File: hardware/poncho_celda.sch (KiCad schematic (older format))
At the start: 0 parts

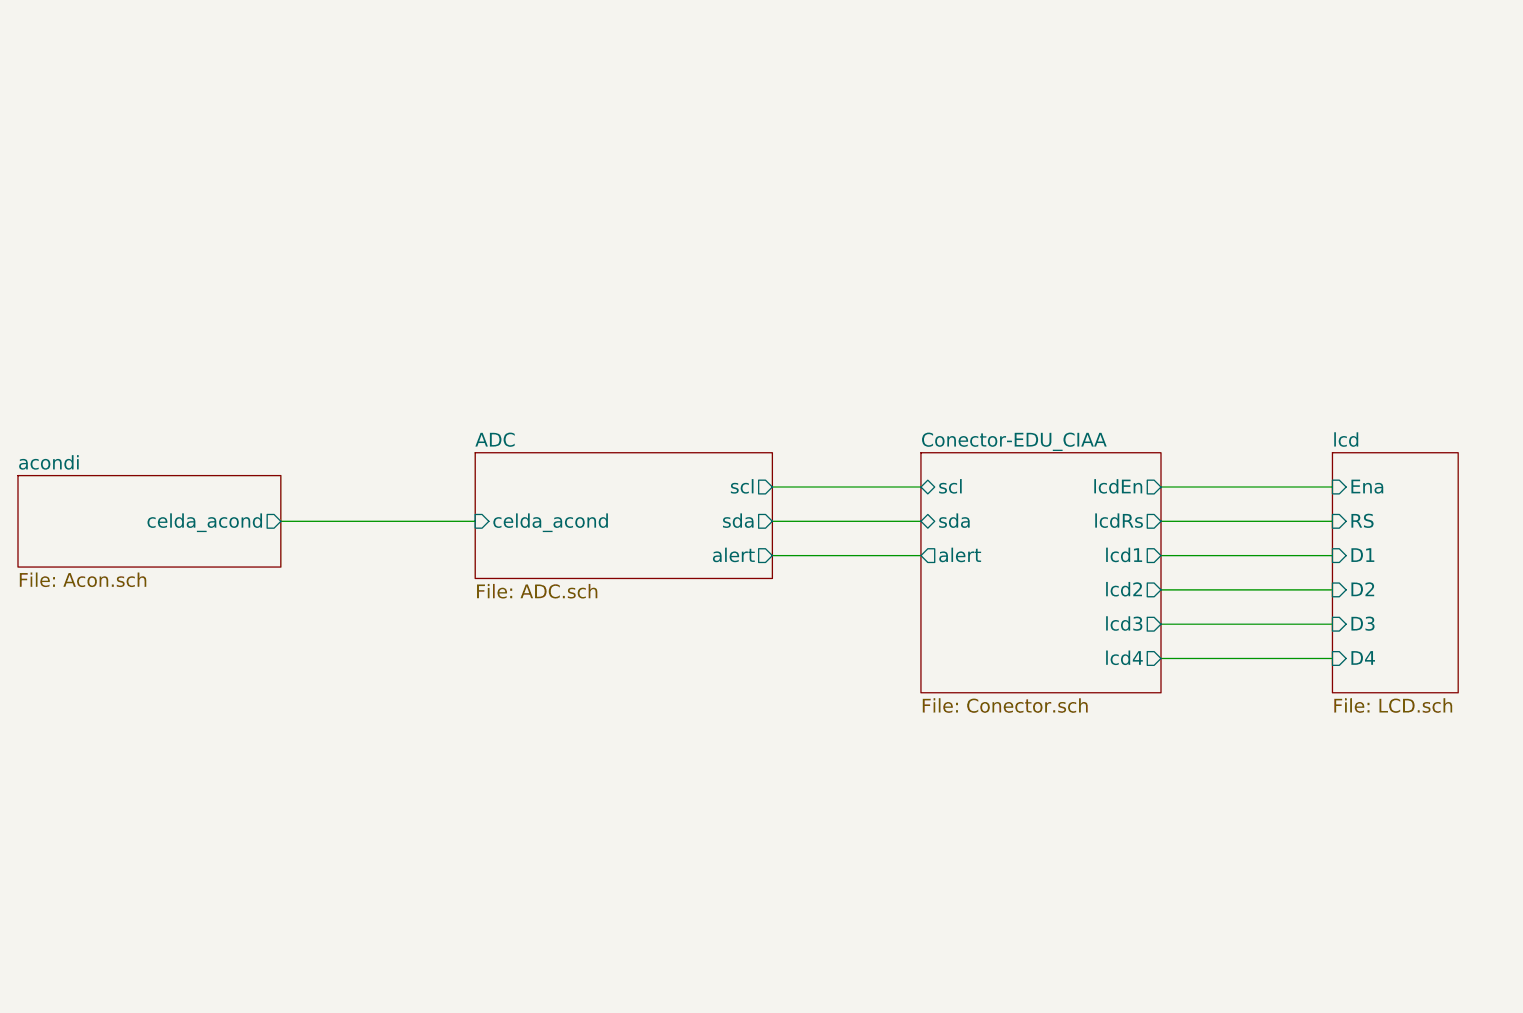
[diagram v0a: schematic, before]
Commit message: Se realizan correcciones al esquematico.
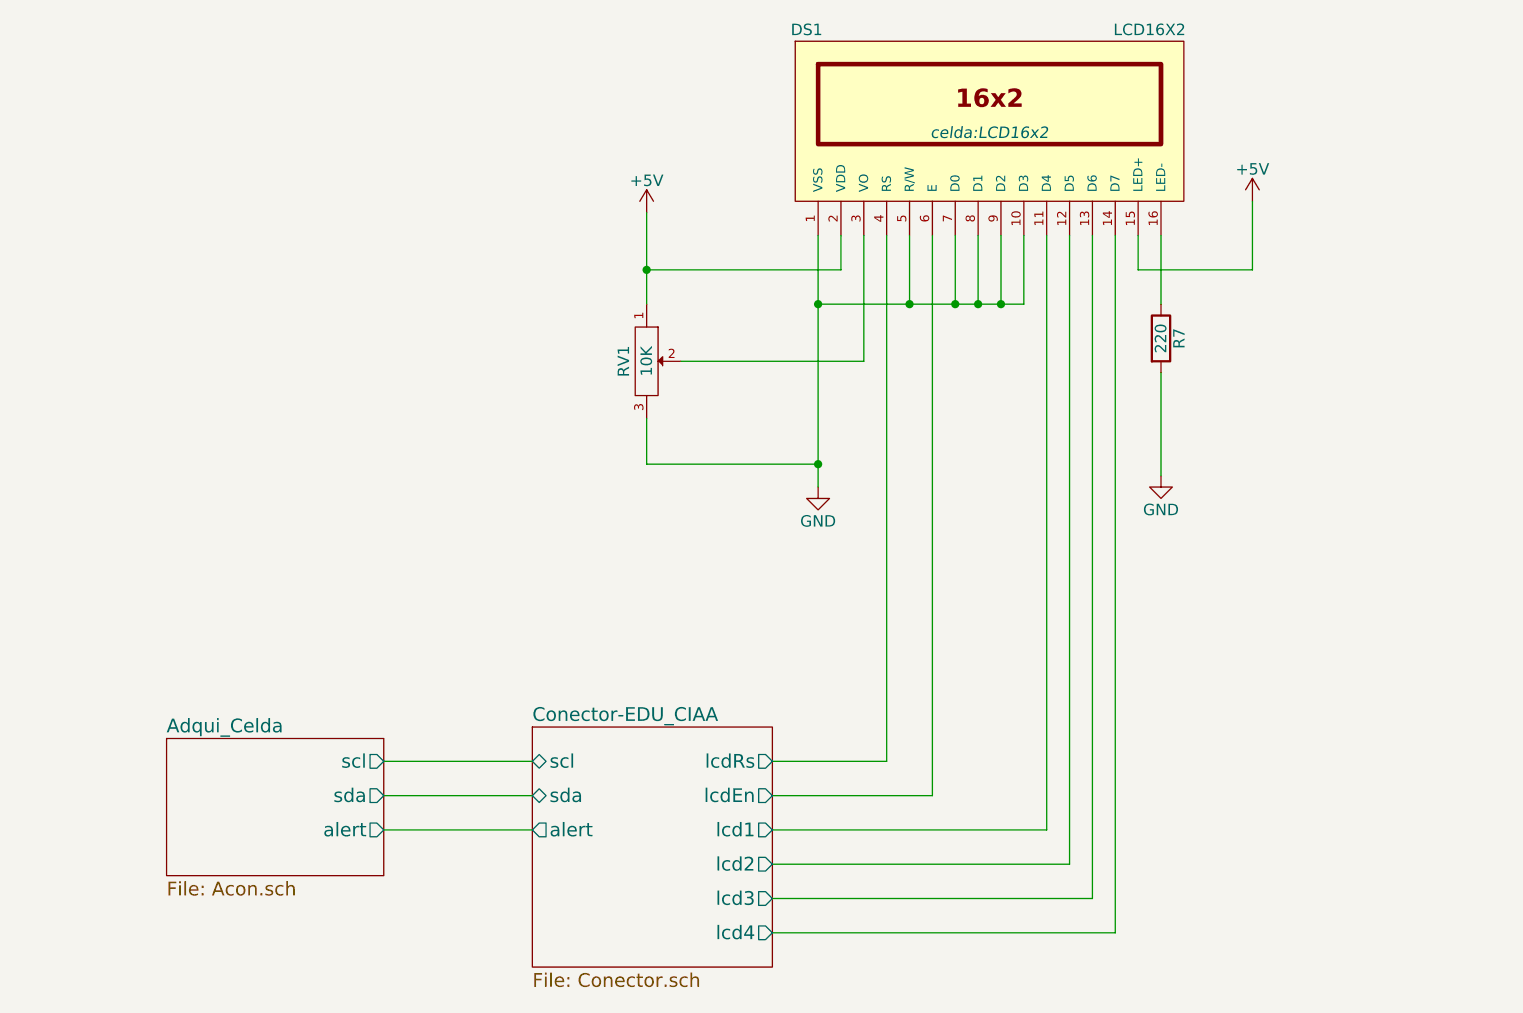
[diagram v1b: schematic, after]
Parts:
- added DS1: LCD16X2, celda:LCD16x2, symbol LCD16X2
- added R7: 220, celda:R_1206_HandSoldering, symbol R
- added RV1: 10K, celda:POT_SMD, symbol POT
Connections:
- net Conector-EDU_CIAA/lcd1: now also DS1.11 (D4)
- net Conector-EDU_CIAA/lcd2: now also DS1.12 (D5)
- net Conector-EDU_CIAA/lcd3: now also DS1.13 (D6)
- net Conector-EDU_CIAA/lcd4: now also DS1.14 (D7)
- net Conector-EDU_CIAA/lcdEn: now also DS1.6 (E)
- net Conector-EDU_CIAA/lcdRs: now also DS1.4 (RS)
- new net: DS1.16 (LED-), R7.1
- new net: DS1.3 (VO), RV1.2
- new net +5V: DS1.15 (LED+), DS1.2 (VDD), RV1.1
- new net GND: DS1.1 (VSS), DS1.10 (D3), DS1.5 (R/W), DS1.7 (D0), DS1.8 (D1), DS1.9 (D2), R7.2, RV1.3
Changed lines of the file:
@@
 $Descr A4 11693 8268
 encoding utf-8
-Sheet 1 5
-Title "Diagrama esquematico de modulos para poncho celda."
+Sheet 1 3
+Title "Diagrama esquematico de poncho Celda."
 Date "2016-07-04"
 Rev ""
 Comp "Felipe Rey"
-Comment1 ""
-Comment2 ""
+Comment1 "Diagrama esquematico de modulos para poncho celda para el curso de Diseño de PCB del CESE."
+Comment2 "Licencia GPL V3"
 Comment3 ""
 Comment4 ""
 $EndDescr
 $Sheet
-S 4350 3250 1300 550
-U 57856888
-F0 "ADC" 60
-F1 "ADC.sch" 60
-F2 "celda_acond" I L 4350 3550 60
-F3 "scl" O R 5650 3400 60
-F4 "sda" O R 5650 3550 60
-F5 "alert" O R 5650 3700 60
+S 3000 4500 950  600
+U 578568AB
+F0 "Adqui_Celda" 60
+F1 "Acon.sch" 60
+F2 "scl" O R 3950 4600 60
+F3 "sda" O R 3950 4750 60
+F4 "alert" O R 3950 4900 60
 $EndSheet
 $Sheet
-S 2350 3350 1150 400
-U 578568AB
-F0 "acondi" 60
-F1 "Acon.sch" 60
-F2 "celda_acond" O R 3500 3550 60
-$EndSheet
-$Sheet
-S 8100 3250 550  1050
-U 578568C8
-F0 "lcd" 60
-F1 "LCD.sch" 60
-F2 "RS" I L 8100 3550 60
-F3 "Ena" I L 8100 3400 60
-F4 "D1" I L 8100 3700 60
-F5 "D2" I L 8100 3850 60
-F6 "D3" I L 8100 4000 60
-F7 "D4" I L 8100 4150 60
-$EndSheet
-$Sheet
-S 6300 3250 1050 1050
+S 4600 4450 1050 1050
 U 578568DA
 F0 "Conector-EDU_CIAA" 60
 F1 "Conector.sch" 60
-F2 "sda" B L 6300 3550 60
-F3 "scl" B L 6300 3400 60
-F4 "lcdEn" O R 7350 3400 60
-F5 "lcdRs" O R 7350 3550 60
-F6 "lcd1" O R 7350 3700 60
-F7 "lcd2" O R 7350 3850 60
-F8 "lcd3" O R 7350 4000 60
-F9 "lcd4" O R 7350 4150 60
-F10 "alert" O L 6300 3700 60
+F2 "sda" B L 4600 4750 60
+F3 "scl" B L 4600 4600 60
+F4 "lcdEn" O R 5650 4750 60
+F5 "lcdRs" O R 5650 4600 60
+F6 "lcd1" O R 5650 4900 60
+F7 "lcd2" O R 5650 5050 60
+F8 "lcd3" O R 5650 5200 60
+F9 "lcd4" O R 5650 5350 60
+F10 "alert" O L 4600 4900 60
 $EndSheet
 Wire Wire Line
-	3500 3550 4350 3550
+	3950 4600 4600 4600
 Wire Wire Line
-	5650 3400 6300 3400
+	3950 4750 4600 4750
 Wire Wire Line
-	5650 3550 6300 3550
+	3950 4900 4600 4900
+$Comp
+L LCD16X2 DS1
+U 1 1 5796E83B
+P 6600 1800
+F 0 "DS1" H 5800 2200 50  0000 C CNN
+F 1 "LCD16X2" H 7300 2200 50  0000 C CNN
+F 2 "celda:LCD16x2" H 6600 1750 50  0000 C CIN
+F 3 "" H 6600 1800 50  0000 C CNN
+	1    6600 1800
+	1    0    0    -1
+$EndComp
+$Comp
+L POT RV1
+U 1 1 5796E97F
+P 5100 2850
+F 0 "RV1" H 5100 2750 50  0000 C CNN
+F 1 "10K" H 5100 2850 50  0000 C CNN
+F 2 "celda:POT_SMD" H 5100 2850 50  0001 C CNN
+F 3 "" H 5100 2850 50  0000 C CNN
+	1    5100 2850
+	0    1    1    0
+$EndComp
+$Comp
+L +5V #PWR01
+U 1 1 5796F4BD
+P 5100 2200
+F 0 "#PWR01" H 5100 2050 50  0001 C CNN
+F 1 "+5V" H 5100 2340 50  0000 C CNN
+F 2 "" H 5100 2200 50  0000 C CNN
+F 3 "" H 5100 2200 50  0000 C CNN
+	1    5100 2200
+	1    0    0    -1
+$EndComp
+$Comp
+L +5V #PWR02
+U 1 1 5796F541
+P 7750 2150
+F 0 "#PWR02" H 7750 2000 50  0001 C CNN
+F 1 "+5V" H 7750 2290 50  0000 C CNN
+F 2 "" H 7750 2150 50  0000 C CNN
+F 3 "" H 7750 2150 50  0000 C CNN
+	1    7750 2150
+	1    0    0    -1
+$EndComp
+$Comp
+L R R7
+U 1 1 5796F5C5
+P 7350 2750
+F 0 "R7" V 7430 2750 50  0000 C CNN
+F 1 "220" V 7350 2750 50  0000 C CNN
+F 2 "celda:R_1206_HandSoldering" V 7280 2750 50  0001 C CNN
+F 3 "" H 7350 2750 50  0000 C CNN
+	1    7350 2750
+	1    0    0    -1
+$EndComp
 Wire Wire Line
-	5650 3700 6300 3700
+	7350 2300 7350 2600
 Wire Wire Line
-	7350 3400 8100 3400
+	7250 2300 7250 2450
 Wire Wire Line
-	8100 3550 7350 3550
+	7250 2450 7750 2450
 Wire Wire Line
-	8100 3700 7350 3700
+	7750 2450 7750 2150
 Wire Wire Line
-	8100 3850 7350 3850
+	5950 2300 5950 2450
 Wire Wire Line
-	8100 4000 7350 4000
+	5950 2450 5100 2450
 Wire Wire Line
-	8100 4150 7350 4150
+	5100 2200 5100 2600
+Connection ~ 5100 2450
+Wire Wire Line
+	6050 2300 6050 2850
+Wire Wire Line
+	6050 2850 5250 2850
+$Comp
+L GND #PWR03
+U 1 1 5796F813
+P 5850 3400
+F 0 "#PWR03" H 5850 3150 50  0001 C CNN
+F 1 "GND" H 5850 3250 50  0000 C CNN
+F 2 "" H 5850 3400 50  0000 C CNN
+F 3 "" H 5850 3400 50  0000 C CNN
+	1    5850 3400
+	1    0    0    -1
+$EndComp
+$Comp
+L GND #PWR04
+U 1 1 5796F899
+P 7350 3350
+F 0 "#PWR04" H 7350 3100 50  0001 C CNN
+F 1 "GND" H 7350 3200 50  0000 C CNN
+F 2 "" H 7350 3350 50  0000 C CNN
+F 3 "" H 7350 3350 50  0000 C CNN
+	1    7350 3350
+	1    0    0    -1
+$EndComp
+Wire Wire Line
+	7350 2900 7350 3350
+Wire Wire Line
+	5850 2300 5850 3400
+Wire Wire Line
+	5100 3100 5100 3300
+Wire Wire Line
+	5100 3300 5850 3300
+Connection ~ 5850 3300
+Wire Wire Line
+	6250 2300 6250 2600
+Wire Wire Line
+	5850 2600 6750 2600
+Connection ~ 5850 2600
+Wire Wire Line
+	6450 2600 6450 2300
+Connection ~ 6250 2600
+Wire Wire Line
+	6550 2600 6550 2300
+Connection ~ 6450 2600
+Wire Wire Line
+	6650 2600 6650 2300
+Connection ~ 6550 2600
+Wire Wire Line
+	6750 2600 6750 2300
+Connection ~ 6650 2600
+Wire Wire Line
+	5650 4600 6150 4600
+Wire Wire Line
+	6150 4600 6150 2300
+Wire Wire Line
+	5650 4750 6350 4750
+Wire Wire Line
+	6350 4750 6350 2300
+Wire Wire Line
+	5650 4900 6850 4900
+Wire Wire Line
+	6850 4900 6850 2300
+Wire Wire Line
+	5650 5050 6950 5050
+Wire Wire Line
+	6950 5050 6950 2300
+Wire Wire Line
+	5650 5200 7050 5200
+Wire Wire Line
+	7050 5200 7050 2300
+Wire Wire Line
+	5650 5350 7150 5350
+Wire Wire Line
+	7150 5350 7150 2300
 $EndSCHEMATC
